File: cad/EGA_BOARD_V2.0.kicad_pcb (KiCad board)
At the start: 2 copper layers, 73 x 60 mm, 14 parts, among them SW1 SWITCH (B3F-1020), SW2 SWITCH (B3F-1020), SW3 SWITCH (B3F-1020)

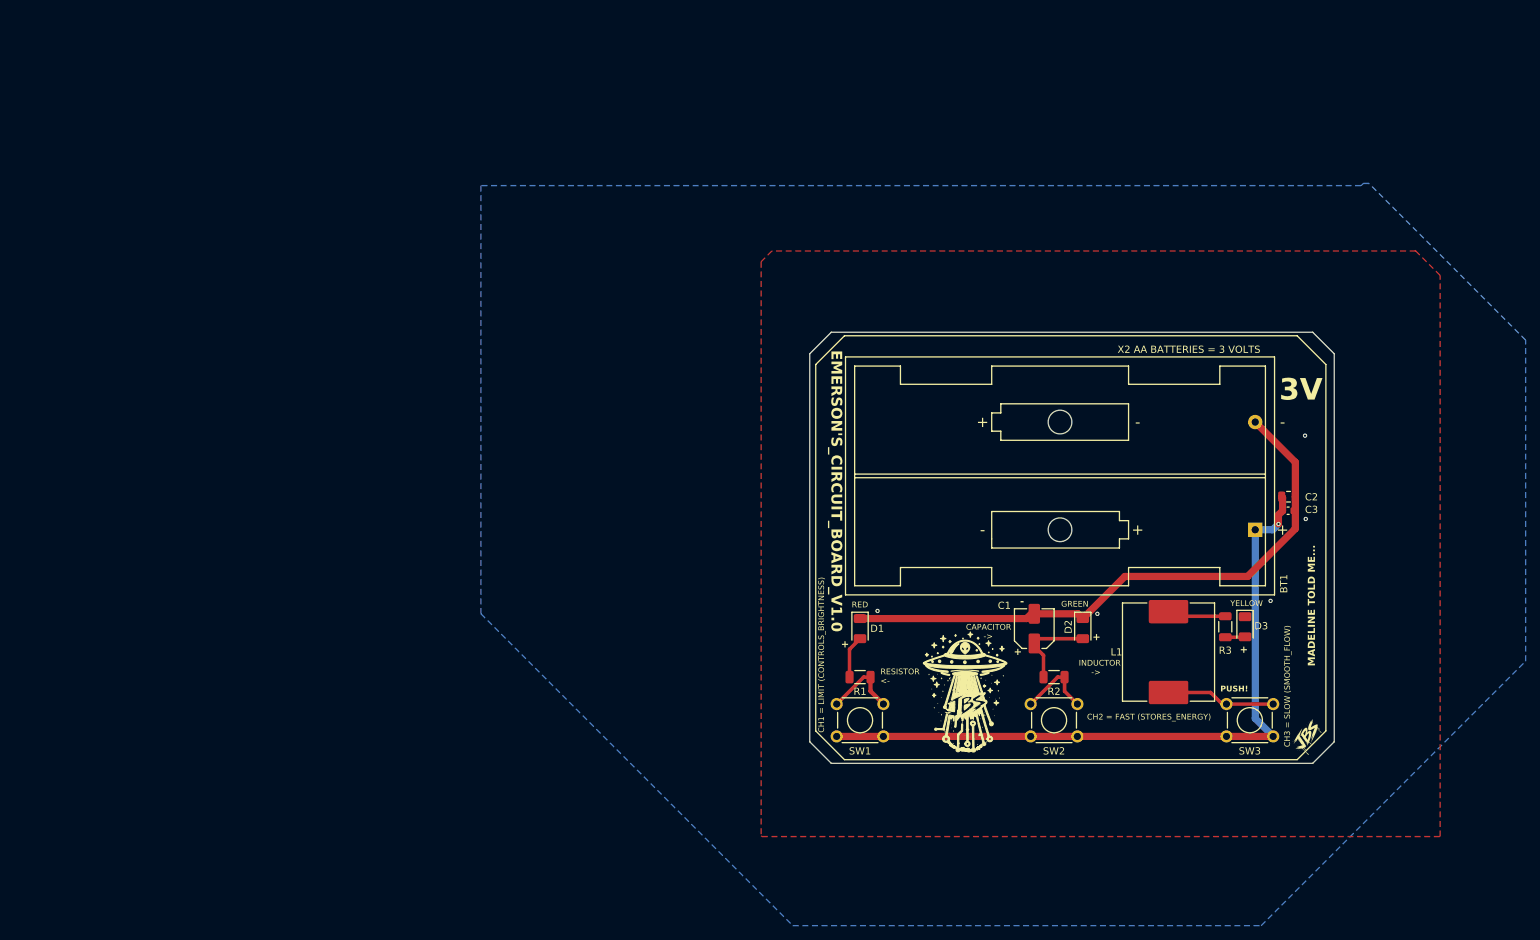
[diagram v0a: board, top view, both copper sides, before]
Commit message: EDITED BOARD
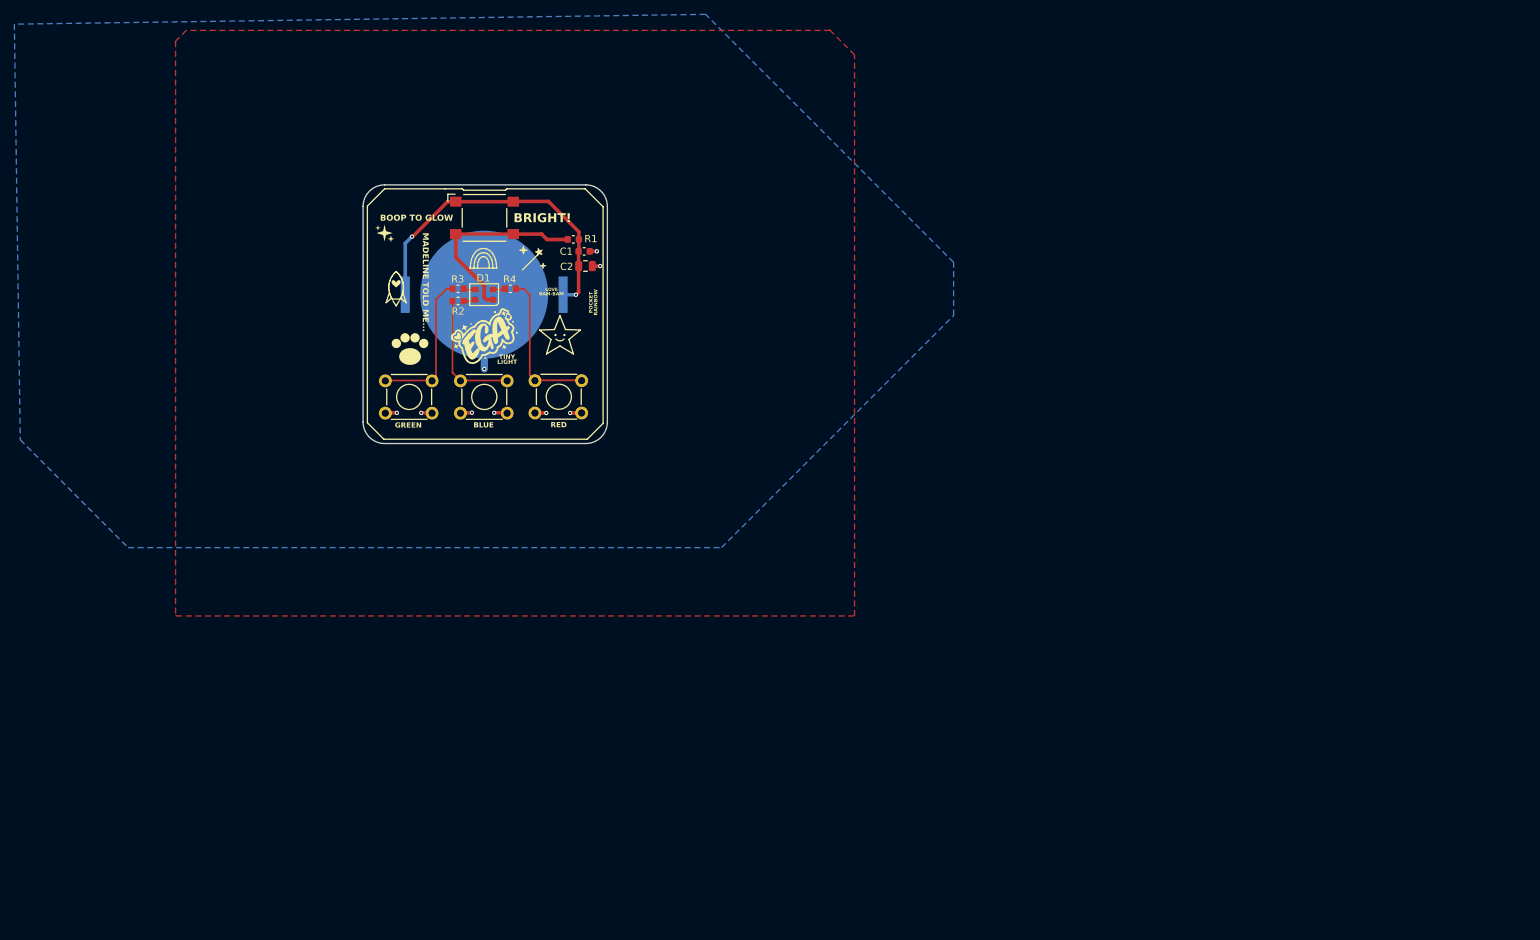
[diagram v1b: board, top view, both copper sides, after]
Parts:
- removed C3: 0.1uF (0603), Capacitor_SMD:C_0603_1608Metric
- removed D2, D3: LED (IR26-21C/L110/TR8), LED_SMD:LED_1206_3216Metric
- removed L1: 47uH (MWSA1206S-470MT), Inductor_SMD:L_Sunlord_MWSA1206S-3R3
- added R4: 1K, CAPS:C_0603_1608Metric, F.Cu at (135.5, 98.5)
- added SW4: SWITCH (B3F-1020), SWITCH_BUTTON:OMRON_SW_THT, F.Cu at (142.2, 113.5)
- BT1: value 3.0V (36-2462-ND) -> 1057; footprint Battery:BatteryHolder_Keystone_2462_2xAA -> Battery:BatteryHolder_Keystone_3034_1x20mm; moved to B.Cu
- C1: value 100uF (EEE-FH1E101XL) -> 100N; footprint Capacitor_SMD:C_Elec_5x5.8 -> CAPS:C_0603_1608Metric
- C2: value 47uF (0805) -> 10U; footprint Capacitor_SMD:C_0805_2012Metric -> CAPS:C_0805_2012Metric
- D1: value LED (IR26-21C/L110/TR8) -> RBG_LED; footprint LED_SMD:LED_1206_3216Metric -> LED:LED_Cree-PLCC4_3.2x2.8mm_CCW
- R1: value 100 (RMCF1206FT100R) -> 2.2K; footprint Resistor_SMD:R_1206_3216Metric -> CAPS:C_0603_1608Metric
- R2: value 100 (RMCF1206FT100R) -> 4.7K; footprint Resistor_SMD:R_1206_3216Metric -> CAPS:C_0603_1608Metric
- R3: value 220 (RMCF1206FT220R) -> 4.7K; footprint Resistor_SMD:R_1206_3216Metric -> CAPS:C_0603_1608Metric
- SW1: value SWITCH (B3F-1020) -> BRIGHT; footprint Button_Switch_THT:SW_TH_Tactile_Omron_B3F-102x -> BUTTON_SWITCH:SW_SPST_Omron_B3FS-100xP
- SW2, SW3: footprint Button_Switch_THT:SW_TH_Tactile_Omron_B3F-102x -> SWITCH_BUTTON:OMRON_SW_THT
- moved SW3 129.3 mm to (121.3, 113.5), turned to 0 degrees
- moved R3 116.7 mm to (128.2, 98.5), turned to 180 degrees
- moved BT1 112.2 mm to (131.9, 99.3)
- moved C2 103.0 mm to (146.0, 95.3)
- moved R2 98.1 mm to (128.2, 100.2), turned to 180 degrees
- moved SW2 95.2 mm to (131.8, 113.5), turned to 0 degrees
- moved SW1 91.0 mm to (131.9, 88.6), turned to 0 degrees
- moved C1 81.7 mm to (145.8, 93.3), turned to 0 degrees
- moved R1 72.8 mm to (144.3, 91.6)
- moved D1 70.0 mm to (131.8, 99.3), turned to 180 degrees
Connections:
- BT1 pad 1: V_IN -> /V_IN
- C1 pad 1: Net-(D2-A) -> /V_IN
- C2 pad 1: V_IN -> /V_IN
- D1 pad 1: GND -> /BRIGHT
- D1 pad 2: Net-(D1-A) -> Net-(D1-RK)
- R1 pad 1: Net-(D1-A) -> /BRIGHT
- R1 pad 2: Net-(R1-Pad2) -> /V_IN
- R2 pad 1: Net-(D2-A) -> Net-(D1-BK)
- R2 pad 2: Net-(R2-Pad2) -> /BLUE
- R3 pad 1: Net-(D3-A) -> Net-(D1-GK)
- R3 pad 2: Net-(L1-Pad2) -> /GREEN
- SW1 pad 1: V_IN -> /V_IN
- SW1 pad 2: Net-(R1-Pad2) -> /BRIGHT
- SW2 pad 1: V_IN -> /BLUE
- SW2 pad 2: Net-(R2-Pad2) -> GND
- SW3 pad 1: V_IN -> /GREEN
- SW3 pad 2: Net-(L1-Pad1) -> GND
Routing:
- net V_IN: track 98.6 -> 0.00 mm, vias 1 -> 0
- net GND: track 83.3 -> 22.2 mm, vias 5 -> 9
- net /V_IN: track 0.00 -> 46.2 mm, vias 0 -> 2
- net /BRIGHT: track 0.00 -> 28.1 mm
- net /RED: track 0.00 -> 21.0 mm
- net /GREEN: track 0.00 -> 21.0 mm
- net /BLUE: track 0.00 -> 18.1 mm
- net Net-(L1-Pad1): track 15.2 -> 0.00 mm
- net Net-(D2-A): track 12.2 -> 0.00 mm
- net Net-(R1-Pad2): track 11.3 -> 0.00 mm
- net Net-(R2-Pad2): track 10.8 -> 0.00 mm
- net Net-(L1-Pad2): track 8.16 -> 0.00 mm
- net Net-(D1-A): track 5.96 -> 0.00 mm
- net Net-(D3-A): track 2.78 -> 0.00 mm
- net Net-(D1-BK): track 0.00 -> 1.67 mm
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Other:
- board size 73 x 60 mm -> 34 x 36 mm
- board text added: "SIGNAL_PLAYGROUND_NANO_V2"
- board text removed: "-"
- board text removed: "CAPACITOR ->"
- board text removed: "CH1 = LIMIT (CONTROLS_BRIGHTNESS)"
- board text removed: "CH2 = FAST (STORES_ENERGY)"
- board text removed: "CH3 = SLOW (SMOOTH_FLOW)"
- board text removed: "EMERSON'S_CIRCUIT_BOARD_V1.0"
- board text removed: "GREEN"
- board text removed: "INDUCTOR ->"
- board text removed: "LOVE, BAM-BAM"
- board text removed: "MADELINE TOLD ME..."
- board text removed: "PUSH!"
- board text removed: "RED"
- board text removed: "RESISTOR <-"
- board text removed: "WHERE'S MAMA...?"
- board text removed: "X2 AA BATTERIES = 3 VOLTS"
- board text removed: "YELLOW"
